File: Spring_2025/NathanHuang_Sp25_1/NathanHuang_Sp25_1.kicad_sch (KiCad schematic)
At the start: 19 parts, among them J1 Barrel_Jack, M1 Motor_Servo, M2 Motor_Servo, M3 Motor_Servo, M4 Motor_Servo, M5 Motor_Servo, M6 Motor_Servo, M7 Stepper_Motor_bipolar, SW1 SW_Push, SW2 SW_Push, U2 LM2596_BUCK_CONVERTER, U3 ESP32-WROOM-32

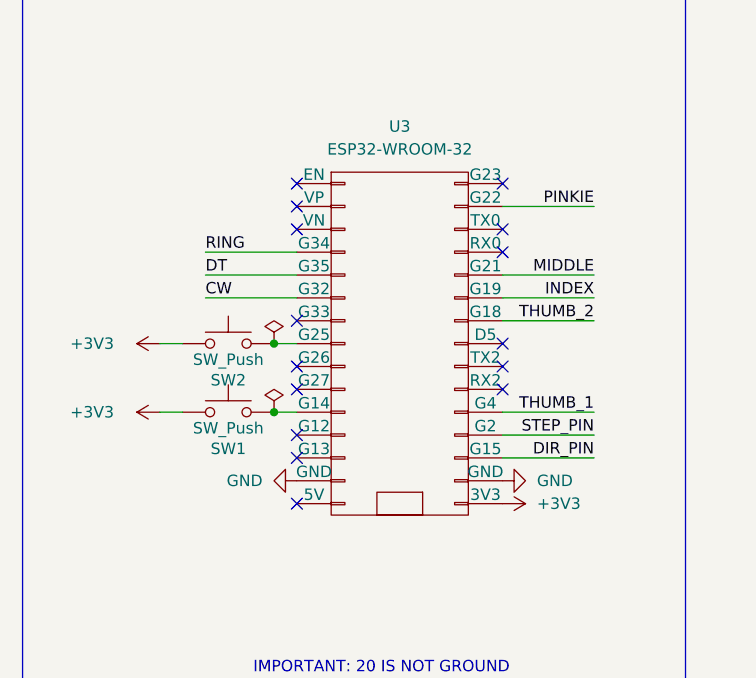
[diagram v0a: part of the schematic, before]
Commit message: Don't clone
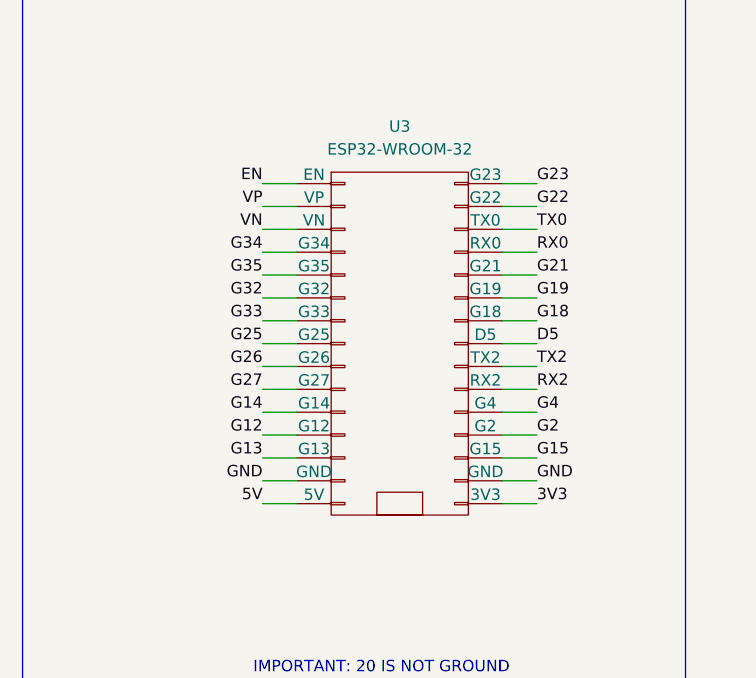
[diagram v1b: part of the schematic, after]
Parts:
- removed SW1, SW2: SW_Push, Connector_PinHeader_2.54mm:PinHeader_1x02_P2.54mm_Vertical, symbol Switch:SW_Push
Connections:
- net +3V3: no longer U3.30 (3V3)
- net CW: no longer U3.6 (G32)
- net DIR_PIN: no longer U3.28 (G15)
- net DT: no longer U3.5 (G35)
- net INDEX: no longer U3.21 (G19)
- net MIDDLE: no longer U3.20 (G21)
- net RING: no longer U3.4 (G34)
- net STEP_PIN: no longer U3.27 (G2)
- net THUMB_1: no longer U3.26 (G4)
- net THUMB_2: no longer U3.22 (G18)
- net G14: now reaches U3.11 (G14)
- net G25: now reaches U3.8 (G25)
- net EN: now reaches U3.1 (EN)
- net G27: now reaches U3.10 (G27)
- net G12: now reaches U3.12 (G12)
- net G13: now reaches U3.13 (G13)
- net 5V: now reaches U3.15 (5V)
- net G23: now reaches U3.16 (G23)
- net TX0: now reaches U3.18 (TX0)
- net RX0: now reaches U3.19 (RX0)
- net VP: now reaches U3.2 (VP)
- net D5: now reaches U3.23 (D5)
- net TX2: now reaches U3.24 (TX2)
- net RX2: now reaches U3.25 (RX2)
- net VN: now reaches U3.3 (VN)
- net G33: now reaches U3.7 (G33)
- net G26: now reaches U3.9 (G26)
- net PINKIE renamed G22
- new net 3V3: U3.30 (3V3)
- new net G15: U3.28 (G15)
- new net G18: U3.22 (G18)
- new net G19: U3.21 (G19)
- new net G2: U3.27 (G2)
- new net G21: U3.20 (G21)
- new net G32: U3.6 (G32)
- new net G34: U3.4 (G34)
- new net G35: U3.5 (G35)
- new net G4: U3.26 (G4)
- no-connect marks 17 -> 2

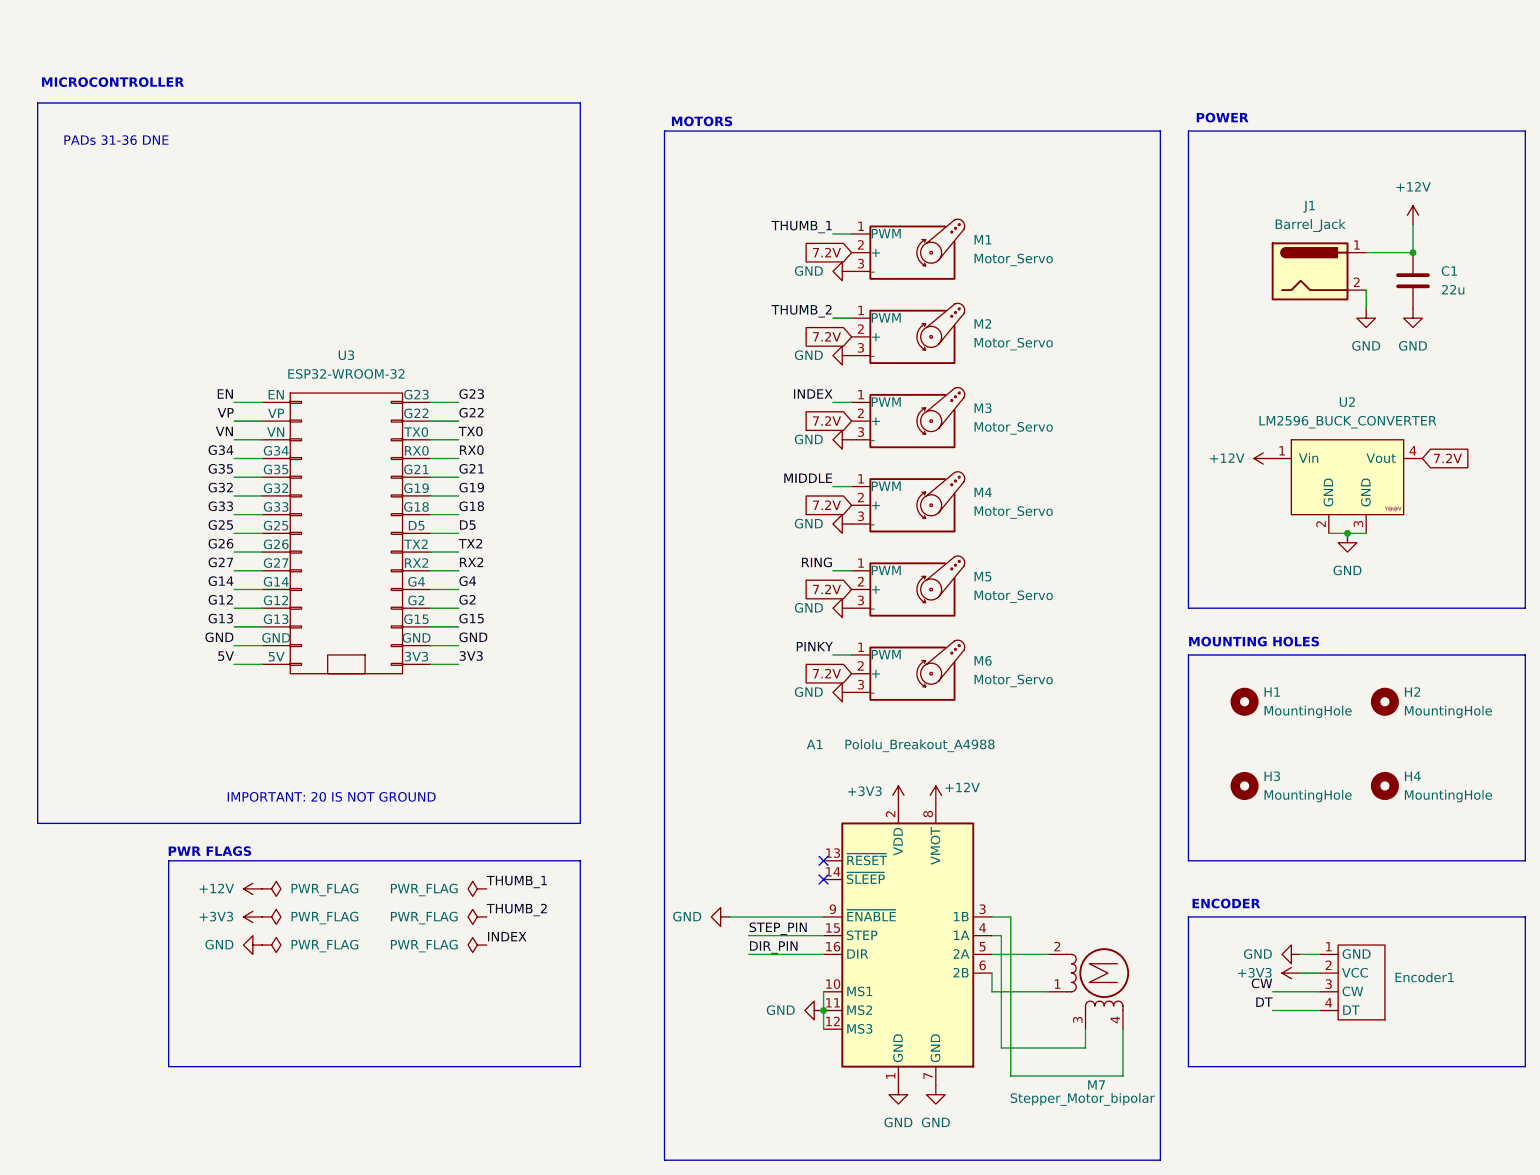
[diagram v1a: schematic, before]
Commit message: Change
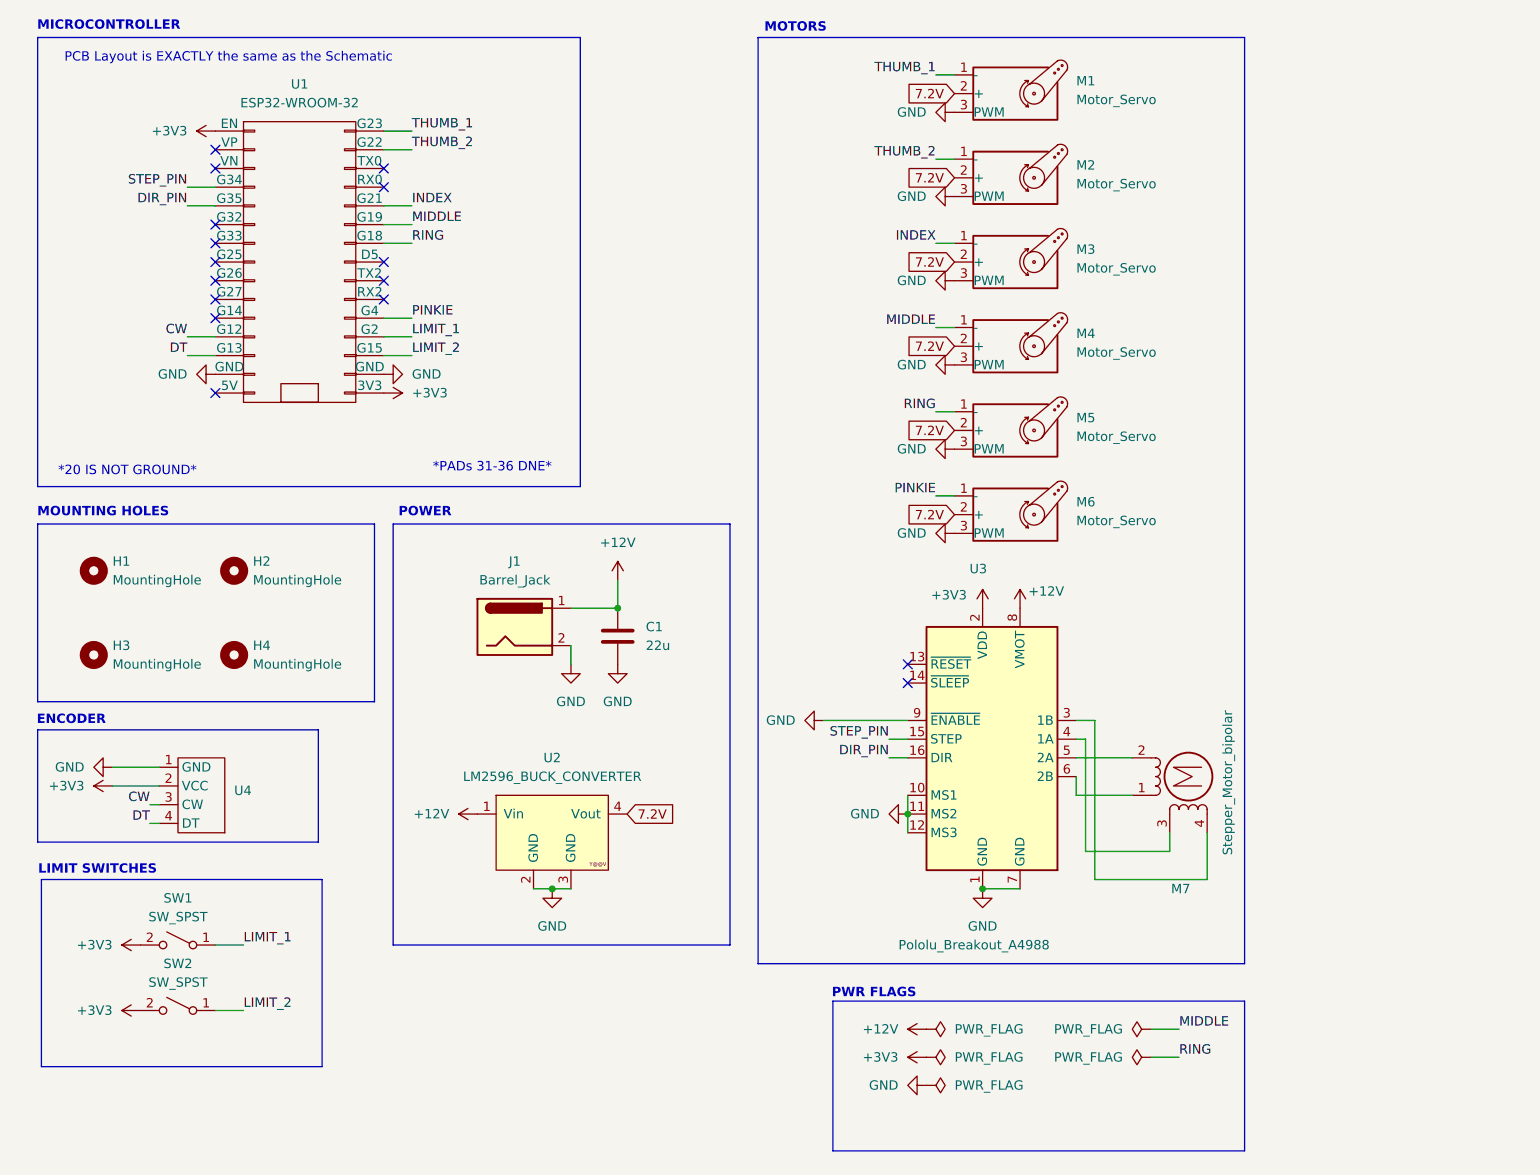
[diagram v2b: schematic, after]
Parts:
- added SW1, SW2: SW_SPST, Connector_PinHeader_2.54mm:PinHeader_1x02_P2.54mm_Vertical, symbol Switch:SW_SPST
- renumbered U3 to U1, A1 to U3, Encoder1 to U4
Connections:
- net 3V3 is gone; now on net +3V3: U1.30 (3V3)
- net EN is gone; now on net +3V3: U1.1 (EN)
- net G12 is gone; now on net CW: U1.12 (G12)
- net G13 is gone; now on net DT: U1.13 (G13)
- net G18 is gone; now on net RING: U1.22 (G18)
- net G19 is gone; now on net MIDDLE: U1.21 (G19)
- net G21 is gone; now on net INDEX: U1.20 (G21)
- net G22 is gone; now on net THUMB_2: U1.17 (G22)
- net G23 is gone; now on net THUMB_1: U1.16 (G23)
- net G34 is gone; now on net STEP_PIN: U1.4 (G34)
- net G35 is gone; now on net DIR_PIN: U1.5 (G35)
- net PINKY is gone; now on net PINKIE: M6.1 (-)
- net +3V3: now also SW1.2 (B), SW2.2 (B)
- net 5V: no longer names the net of U1.15 (5V)
- net D5: no longer names the net of U1.23 (D5)
- net G14: no longer names the net of U1.11 (G14)
- net G15 renamed LIMIT_2
- net LIMIT_2: now also SW2.1 (A)
- net G2 renamed LIMIT_1
- net LIMIT_1: now also SW1.1 (A)
- net G25: no longer names the net of U1.8 (G25)
- net G26: no longer names the net of U1.9 (G26)
- net G27: no longer names the net of U1.10 (G27)
- net G32: no longer names the net of U1.6 (G32)
- net G33: no longer names the net of U1.7 (G33)
- net G4 renamed PINKIE
- net RX0: no longer names the net of U1.19 (RX0)
- net RX2: no longer names the net of U1.25 (RX2)
- net TX0: no longer names the net of U1.18 (TX0)
- net TX2: no longer names the net of U1.24 (TX2)
- net VN: no longer names the net of U1.3 (VN)
- net VP: no longer names the net of U1.2 (VP)
- no-connect marks 2 -> 16
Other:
- note added: "*20 IS NOT GROUND*"
- note added: "*PADs 31-36 DNE*"
- note added: "LIMIT SWITCHES"
- note added: "PCB Layout is EXACTLY the same as the Schematic"
- note removed: "IMPORTANT: 20 IS NOT GROUND"
- note removed: "PADs 31-36 DNE"
- moved on the sheet: C1, H1, H2, H3, H4, J1, M3, M7, U1, U2, U3, U4
